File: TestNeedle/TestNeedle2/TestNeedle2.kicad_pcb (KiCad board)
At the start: 2 copper layers, 13.5 x 78 mm, 3 parts, among them J1 Conn_01x05_Male, J2 Conn_01x05_Male

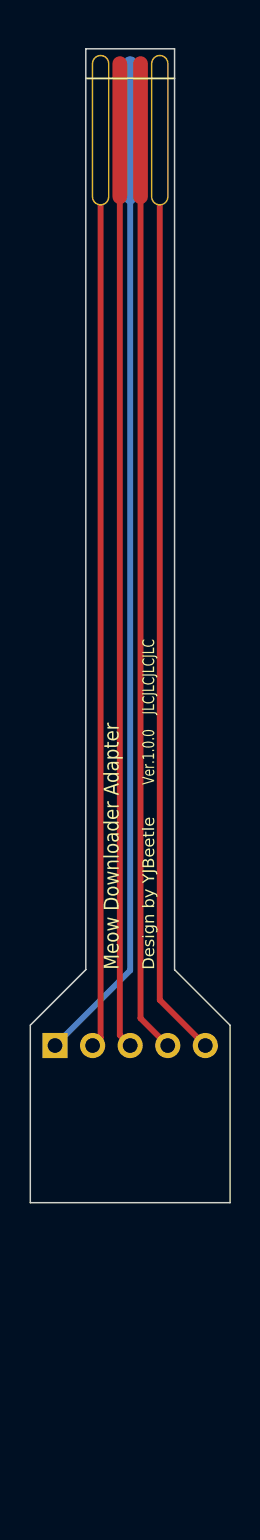
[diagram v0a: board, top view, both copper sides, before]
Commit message: 新设计棒子板
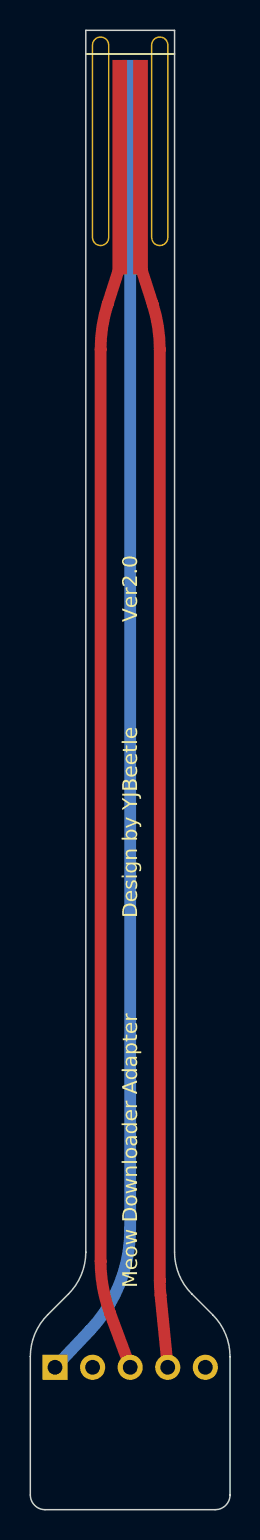
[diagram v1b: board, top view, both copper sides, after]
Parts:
- moved J1 21.8 mm to (137.2, 155.4)
- moved REF** 21.8 mm to (142.2, 157.8)
- moved J2 6.75 mm to (142.2, 65.0)
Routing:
- net Net-(J1-Pin_2): track 62.1 -> 82.9 mm
- net Net-(J1-Pin_5): track 63.2 -> 83.6 mm
- net Net-(J1-Pin_3): track 62.2 -> 81.6 mm
- net Net-(J1-Pin_1): track 64.0 -> 82.7 mm
- net Net-(J1-Pin_4): track 62.6 -> 81.3 mm
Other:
- board size 13.5 x 78 mm -> 13.5 x 100 mm
- copper layers 2 -> 4
- board text added: "V-CUT"
- board text added: "Ver2.0"
- board text removed: "JLCJLCJLCJLC"
- board text removed: "Ver.1.0.0"
